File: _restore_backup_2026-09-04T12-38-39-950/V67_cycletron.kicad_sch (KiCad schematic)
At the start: 49 parts, among them J1 USB_C_Receptacle_USB2.0_16P, J10 Screw_Terminal_01x02, J11 PINHD_1x2_Male, J13 PINHD_2x2_Male, J2 PINHD_1x2_Male, J3 PINHD_1x2_Male, J4 PINHD_1x4_Male, J5 PINHD_1x4_Male, J6 PINHD_1x4_Male, J7 PINHD_1x4_Male, J8 PINHD_2x4_Male, J9 PINHD_1x3_Male, Q1 IRF1324, U2 LM1117DT-3.3, U3 L7805, U4 ESP32-S3-WROOM-1

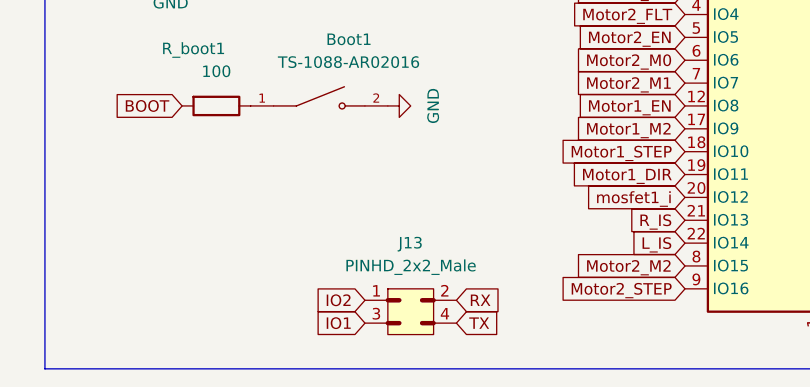
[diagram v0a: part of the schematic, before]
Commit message: big changes to make it work
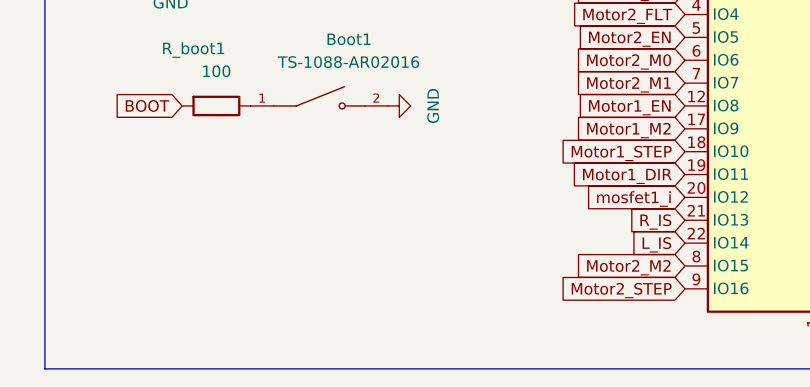
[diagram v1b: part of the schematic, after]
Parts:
- removed J13: PINHD_2x2_Male, Connector_PinHeader_2.54mm:PinHeader_2x02_P2.54mm_Vertical, symbol PCM_SL_Pin_Headers:PINHD_2x2_Male
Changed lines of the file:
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@@
 		)
 	)
-	(global_label "IO1"
-		(shape input)
-		(at 60.96 189.23 180)
-		(fields_autoplaced yes)
-		(effects
-			(font
-				(size 1.27 1.27)
-			)
-			(justify right)
-		)
-		(property "Intersheetrefs" "${INTERSHEET_REFS}"
-			(at 54.83 189.23 0)
-			(hide yes)
-			(show_name no)
-			(do_not_autoplace no)
-			(effects
-				(font
-					(size 1.27 1.27)
-				)
-				(justify right)
-			)
-		)
-	)
 	(global_label "Motor1_M2"
 		(shape input)
@@
 		)
 	)
-	(global_label "TX"
-		(shape input)
-		(at 71.12 189.23 0)
-		(fields_autoplaced yes)
-		(effects
-			(font
-				(size 1.27 1.27)
-			)
-			(justify left)
-		)
-		(property "Intersheetrefs" "${INTERSHEET_REFS}"
-			(at 76.2823 189.23 0)
-			(hide yes)
-			(show_name no)
-			(do_not_autoplace no)
-			(effects
-				(font
-					(size 1.27 1.27)
-				)
-				(justify left)
-			)
-		)
-	)
 	(global_label "Motor2_A1"
 		(shape input)
@@
 		)
 	)
-	(global_label "IO2"
-		(shape input)
-		(at 60.96 186.69 180)
-		(fields_autoplaced yes)
-		(effects
-			(font
-				(size 1.27 1.27)
-			)
-			(justify right)
-		)
-		(property "Intersheetrefs" "${INTERSHEET_REFS}"
-			(at 54.83 186.69 0)
-			(hide yes)
-			(show_name no)
-			(do_not_autoplace no)
-			(effects
-				(font
-					(size 1.27 1.27)
-				)
-				(justify right)
-			)
-		)
-	)
 	(global_label "Motor2_EN"
 		(shape input)
@@
 		)
 	)
-	(global_label "RX"
-		(shape input)
-		(at 71.12 186.69 0)
-		(fields_autoplaced yes)
-		(effects
-			(font
-				(size 1.27 1.27)
-			)
-			(justify left)
-		)
-		(property "Intersheetrefs" "${INTERSHEET_REFS}"
-			(at 76.5847 186.69 0)
-			(hide yes)
-			(show_name no)
-			(do_not_autoplace no)
-			(effects
-				(font
-					(size 1.27 1.27)
-				)
-				(justify left)
-			)
-		)
-	)
 	(global_label "24V_unsafe"
 		(shape input)
@@
 					(unit 1)
 				)
-			)
-		)
-	)
-	(symbol
-		(lib_id "PCM_SL_Pin_Headers:PINHD_2x2_Male")
-		(at 66.04 187.96 0)
-		(unit 1)
-		(body_style 1)
-		(exclude_from_sim no)
-		(in_bom yes)
-		(on_board yes)
-		(in_pos_files yes)
-		(dnp no)
-		(fields_autoplaced yes)
-		(property "Reference" "J13"
-			(at 66.04 180.34 0)
-			(show_name no)
-			(do_not_autoplace no)
-			(effects
-				(font
-					(size 1.27 1.27)
-				)
-			)
-		)
-		(property "Value" "PINHD_2x2_Male"
-			(at 66.04 182.88 0)
-			(show_name no)
-			(do_not_autoplace no)
-			(effects
-				(font
-					(size 1.27 1.27)
-				)
-			)
-		)
-		(property "Footprint" "Connector_PinHeader_2.54mm:PinHeader_2x02_P2.54mm_Vertical"
-			(at 66.04 191.77 0)
-			(hide yes)
-			(show_name no)
-			(do_not_autoplace no)
-			(effects
-				(font
-					(size 1.27 1.27)
-				)
-			)
-		)
-		(property "Datasheet" ""
-			(at 64.77 180.34 0)
-			(hide yes)
-			(show_name no)
-			(do_not_autoplace no)
-			(effects
-				(font
-					(size 1.27 1.27)
-				)
-			)
-		)
-		(property "Description" "Pin Header male with pin space 2.54mm. Pin Count -4"
-			(at 66.04 187.96 0)
-			(hide yes)
-			(show_name no)
-			(do_not_autoplace no)
-			(effects
-				(font
-					(size 1.27 1.27)
-				)
-			)
-		)
-		(pin "2"
-		)
-		(pin "3"
-		)
-		(pin "1"
-		)
-		(pin "4"
-		)
-		(instances
-			(project "V67_cycletron"
-				(path "/490d8b32-3aea-4f11-93e7-a546853a1b13"
-					(reference "J13")
-					(unit 1)
-				)
